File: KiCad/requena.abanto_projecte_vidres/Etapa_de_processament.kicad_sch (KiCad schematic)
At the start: 16 parts, among them U1 PIC24HJ128GP502, U2 NMUX1308PW, Y2 Crystal

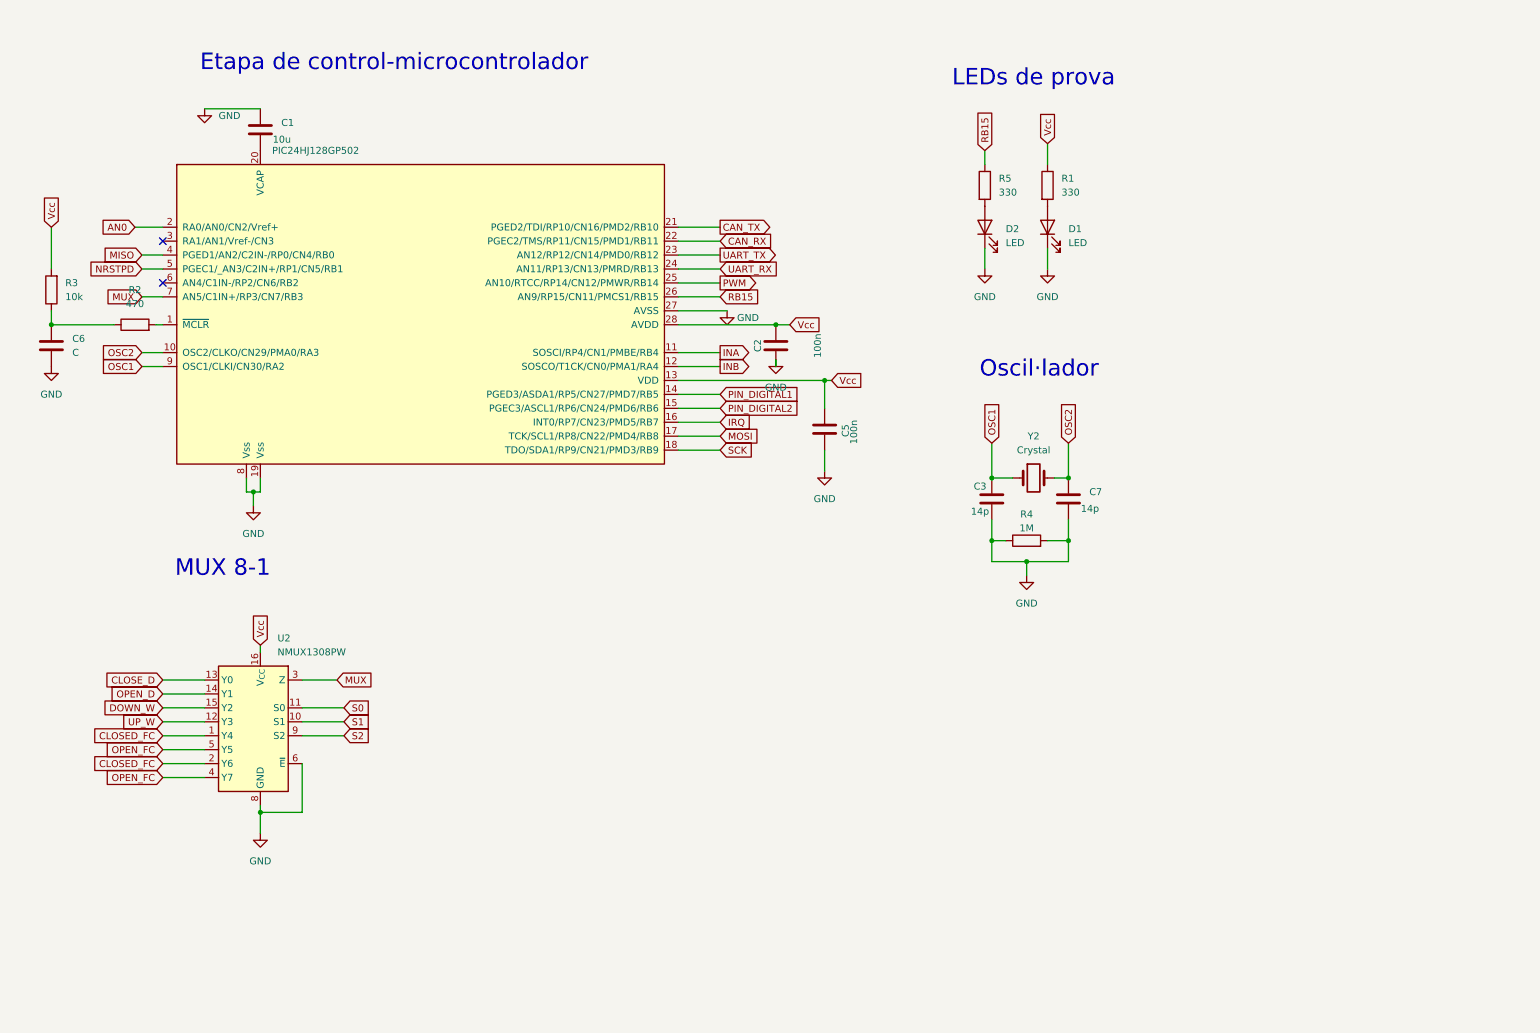
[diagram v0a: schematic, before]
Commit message: Millora projecte 1
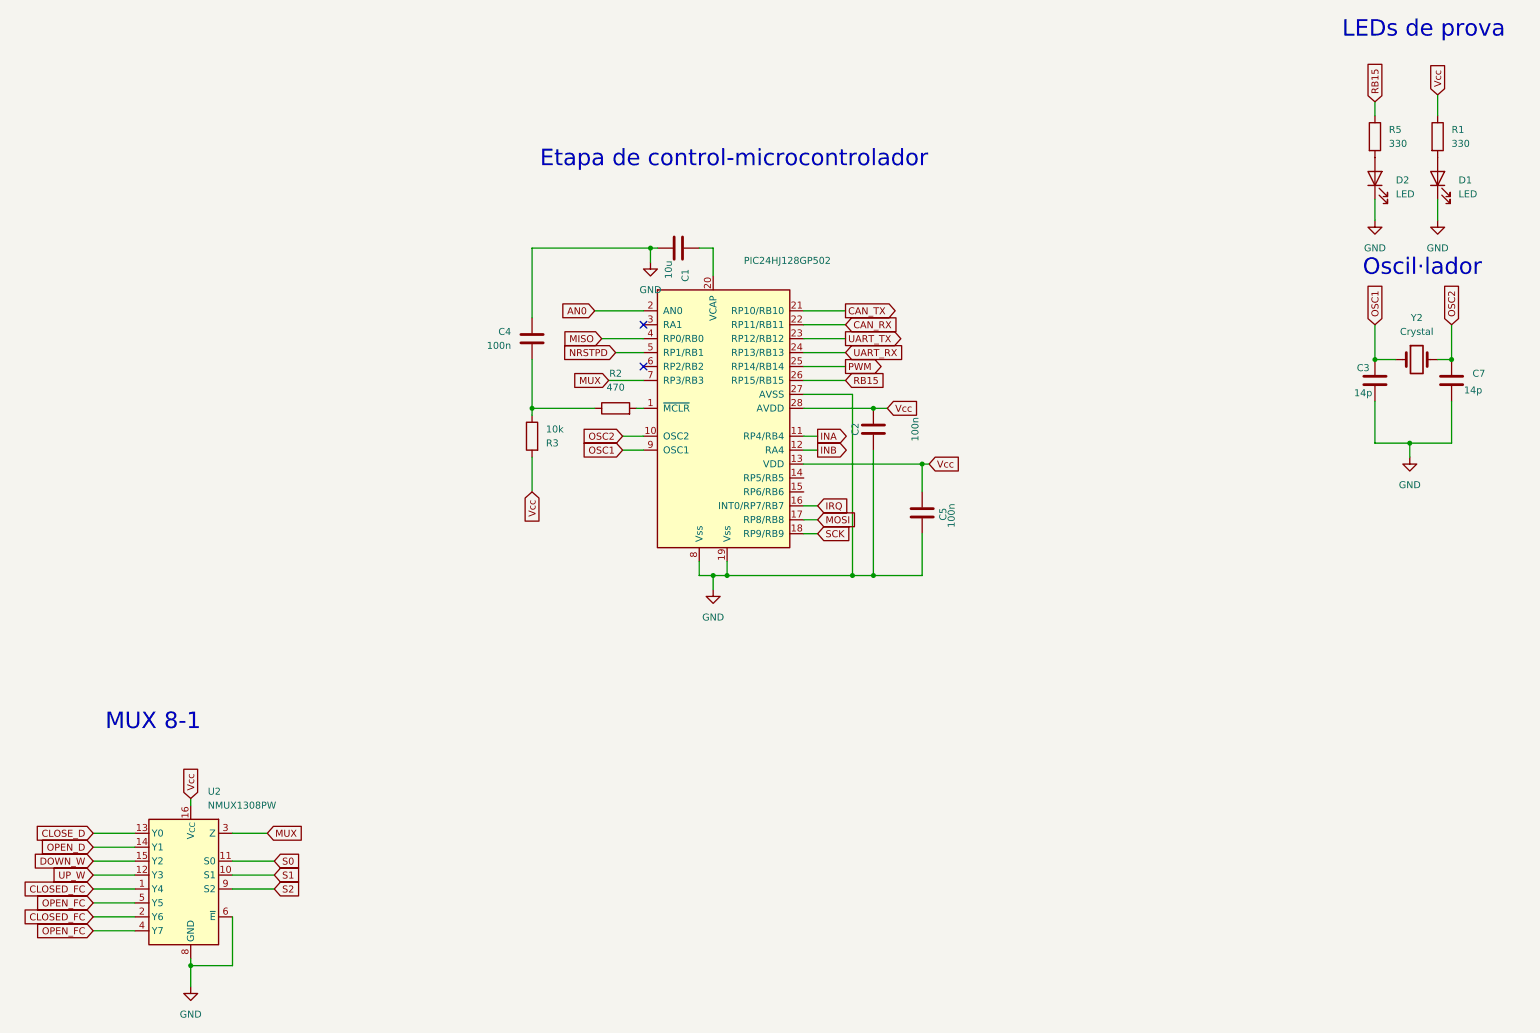
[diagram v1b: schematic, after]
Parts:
- removed C6: C, symbol Device:C
- removed R4: 1M, symbol Device:R
- added C4: 100n, symbol Device:C
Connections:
- net GND: now also C1.2, C4.2; no longer C1.1
- net at R2.1, R3.1: now also C4.1
- net at U1.20 (VCAP): now also C1.1; no longer C1.2
- net PIN_DIGITAL1: no longer names the net of U1.14 (RP5/RB5)
- net PIN_DIGITAL2: no longer names the net of U1.15 (RP6/RB6)
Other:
- moved on the sheet: C1, C2, C3, C5, C7, D1, D2, R1, R2, R3, R5, U2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
